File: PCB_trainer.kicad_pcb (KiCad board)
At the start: 2 copper layers, 76.7 x 55.9 mm, 6 parts, among them IC1 IS42S16800F-7BLI, U1 STM32F103C8Tx, U2 MIMXRT1062DVJ6B, U3 STM32F407VGTx, U4 MIC23158YML-T5, U5 W25Q64JVXGIQ TR

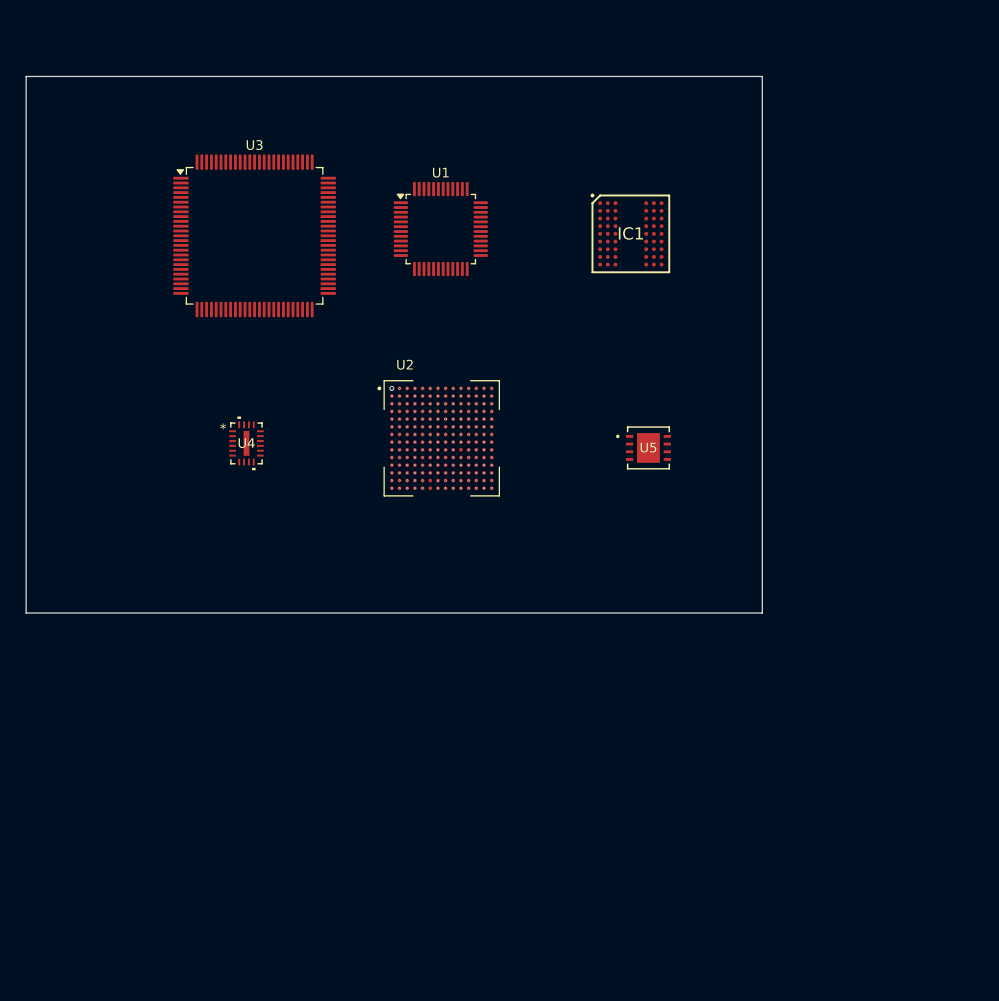
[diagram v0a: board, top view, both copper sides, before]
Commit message: finalised pcb
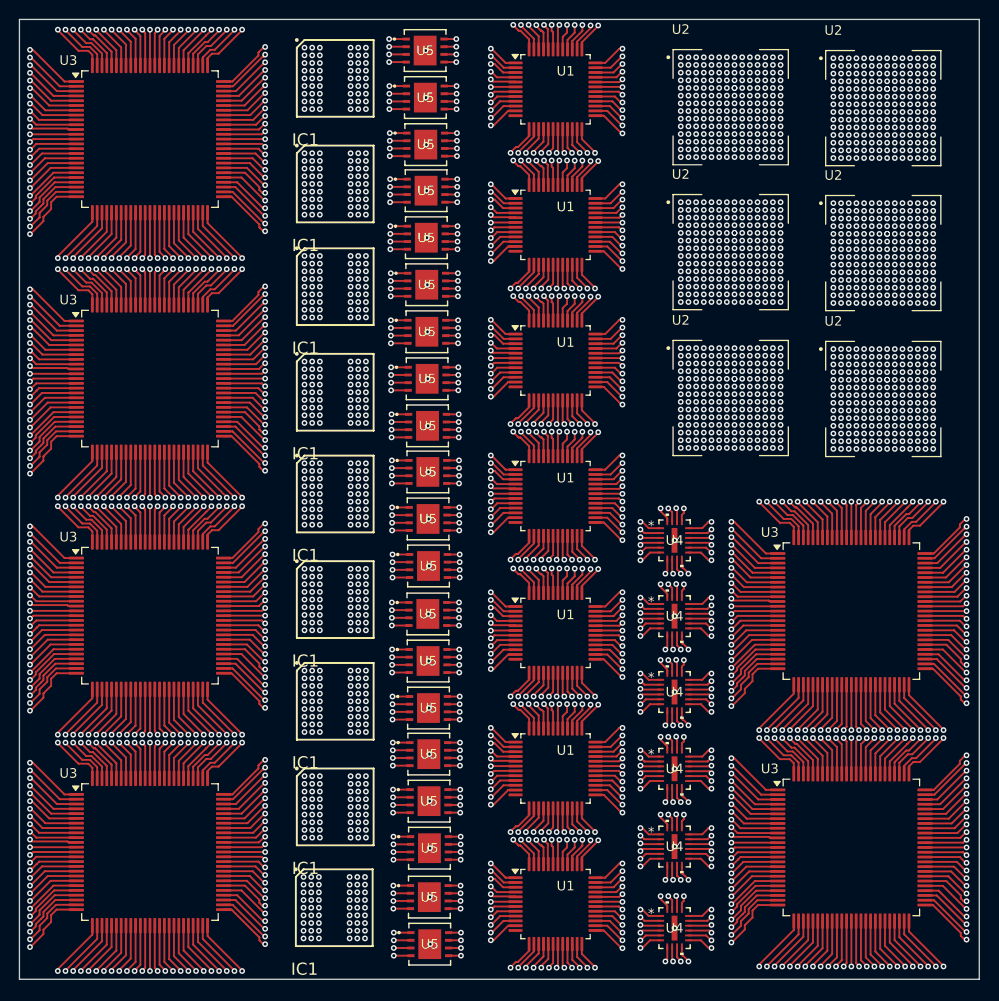
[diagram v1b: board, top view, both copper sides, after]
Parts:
- added IC1: IS42S16800F-7BLI, LIB_IS42S16800F-7BLI:BGA54C80P9X9_800X800X120, F.Cu at (132.9, 110.9)
- added IC1: IS42S16800F-7BLI, LIB_IS42S16800F-7BLI:BGA54C80P9X9_800X800X120, F.Cu at (132.9, 100.3)
- added IC1: IS42S16800F-7BLI, LIB_IS42S16800F-7BLI:BGA54C80P9X9_800X800X120, F.Cu at (132.9, 121.9)
- added IC1: IS42S16800F-7BLI, LIB_IS42S16800F-7BLI:BGA54C80P9X9_800X800X120, F.Cu at (132.9, 78.7)
- added IC1: IS42S16800F-7BLI, LIB_IS42S16800F-7BLI:BGA54C80P9X9_800X800X120, F.Cu at (132.9, 57.0)
- added IC1: IS42S16800F-7BLI, LIB_IS42S16800F-7BLI:BGA54C80P9X9_800X800X120, F.Cu at (132.9, 89.3)
- added IC1: IS42S16800F-7BLI, LIB_IS42S16800F-7BLI:BGA54C80P9X9_800X800X120, F.Cu at (132.8, 132.4)
- added IC1: IS42S16800F-7BLI, LIB_IS42S16800F-7BLI:BGA54C80P9X9_800X800X120, F.Cu at (132.9, 67.7)
- added U1: STM32F103C8Tx, Package_QFP:LQFP-48_7x7mm_P0.5mm, F.Cu at (155.8, 75.4)
- added U1: STM32F103C8Tx, Package_QFP:LQFP-48_7x7mm_P0.5mm, F.Cu at (155.8, 132.0)
- added U1: STM32F103C8Tx, Package_QFP:LQFP-48_7x7mm_P0.5mm, F.Cu at (155.8, 89.5)
- added U1: STM32F103C8Tx, Package_QFP:LQFP-48_7x7mm_P0.5mm, F.Cu at (155.8, 103.8)
- added U1: STM32F103C8Tx, Package_QFP:LQFP-48_7x7mm_P0.5mm, F.Cu at (155.8, 117.9)
- added U1: STM32F103C8Tx, Package_QFP:LQFP-48_7x7mm_P0.5mm, F.Cu at (155.8, 61.3)
- added U2: MIMXRT1062DVJ6B, MIMXRT1062DVJ6B:BGA196C80P14X14_1200X1200X152N, F.Cu at (174.1, 79.3)
- added U2: MIMXRT1062DVJ6B, MIMXRT1062DVJ6B:BGA196C80P14X14_1200X1200X152N, F.Cu at (174.1, 64.1)
- added U2: MIMXRT1062DVJ6B, MIMXRT1062DVJ6B:BGA196C80P14X14_1200X1200X152N, F.Cu at (190.0, 49.1)
- added U2: MIMXRT1062DVJ6B, MIMXRT1062DVJ6B:BGA196C80P14X14_1200X1200X152N, F.Cu at (190.0, 79.4)
- added U2: MIMXRT1062DVJ6B, MIMXRT1062DVJ6B:BGA196C80P14X14_1200X1200X152N, F.Cu at (190.0, 64.2)
- added U3: STM32F407VGTx, Package_QFP:LQFP-100_14x14mm_P0.5mm, F.Cu at (186.7, 101.5)
- added U3: STM32F407VGTx, Package_QFP:LQFP-100_14x14mm_P0.5mm, F.Cu at (186.7, 126.1)
- added U3: STM32F407VGTx, Package_QFP:LQFP-100_14x14mm_P0.5mm, F.Cu at (113.6, 126.6)
- added U3: STM32F407VGTx, Package_QFP:LQFP-100_14x14mm_P0.5mm, F.Cu at (113.6, 77.3)
- added U3: STM32F407VGTx, Package_QFP:LQFP-100_14x14mm_P0.5mm, F.Cu at (113.6, 102.0)
- added U4: MIC23158YML-T5, ul_MIC23158YML-T5:QFN20_3X4_MCH, F.Cu at (168.3, 117.9)
- added U4: MIC23158YML-T5, ul_MIC23158YML-T5:QFN20_3X4_MCH, F.Cu at (168.3, 134.5)
- added U4: MIC23158YML-T5, ul_MIC23158YML-T5:QFN20_3X4_MCH, F.Cu at (168.3, 109.9)
- added U4: MIC23158YML-T5, ul_MIC23158YML-T5:QFN20_3X4_MCH, F.Cu at (168.3, 126.0)
- added U4: MIC23158YML-T5, ul_MIC23158YML-T5:QFN20_3X4_MCH, F.Cu at (168.3, 102.0)
- added U5: W25Q64JVXGIQ TR, ul_W25Q64JVXGIQ-TR:DFN_XGIQ TR_WIN, F.Cu at (142.6, 111.6)
- added U5: W25Q64JVXGIQ TR, ul_W25Q64JVXGIQ-TR:DFN_XGIQ TR_WIN, F.Cu at (142.7, 121.3)
- added U5: W25Q64JVXGIQ TR, ul_W25Q64JVXGIQ-TR:DFN_XGIQ TR_WIN, F.Cu at (142.4, 72.4)
- added U5: W25Q64JVXGIQ TR, ul_W25Q64JVXGIQ-TR:DFN_XGIQ TR_WIN, F.Cu at (142.5, 87.0)
- added U5: W25Q64JVXGIQ TR, ul_W25Q64JVXGIQ-TR:DFN_XGIQ TR_WIN, F.Cu at (142.4, 62.6)
- added U5: W25Q64JVXGIQ TR, ul_W25Q64JVXGIQ-TR:DFN_XGIQ TR_WIN, F.Cu at (142.6, 96.8)
- added U5: W25Q64JVXGIQ TR, ul_W25Q64JVXGIQ-TR:DFN_XGIQ TR_WIN, F.Cu at (142.7, 126.2)
- added U5: W25Q64JVXGIQ TR, ul_W25Q64JVXGIQ-TR:DFN_XGIQ TR_WIN, F.Cu at (142.3, 48.0)
- added U5: W25Q64JVXGIQ TR, ul_W25Q64JVXGIQ-TR:DFN_XGIQ TR_WIN, F.Cu at (142.6, 91.9)
- added U5: W25Q64JVXGIQ TR, ul_W25Q64JVXGIQ-TR:DFN_XGIQ TR_WIN, F.Cu at (142.3, 52.9)
- added U5: W25Q64JVXGIQ TR, ul_W25Q64JVXGIQ-TR:DFN_XGIQ TR_WIN, F.Cu at (142.7, 136.2)
- added U5: W25Q64JVXGIQ TR, ul_W25Q64JVXGIQ-TR:DFN_XGIQ TR_WIN, F.Cu at (142.6, 106.7)
- added U5: W25Q64JVXGIQ TR, ul_W25Q64JVXGIQ-TR:DFN_XGIQ TR_WIN, F.Cu at (142.5, 101.8)
- added U5: W25Q64JVXGIQ TR, ul_W25Q64JVXGIQ-TR:DFN_XGIQ TR_WIN, F.Cu at (142.7, 131.3)
- added U5: W25Q64JVXGIQ TR, ul_W25Q64JVXGIQ-TR:DFN_XGIQ TR_WIN, F.Cu at (142.4, 57.7)
- added U5: W25Q64JVXGIQ TR, ul_W25Q64JVXGIQ-TR:DFN_XGIQ TR_WIN, F.Cu at (142.5, 82.2)
- added U5: W25Q64JVXGIQ TR, ul_W25Q64JVXGIQ-TR:DFN_XGIQ TR_WIN, F.Cu at (142.5, 77.3)
- added U5: W25Q64JVXGIQ TR, ul_W25Q64JVXGIQ-TR:DFN_XGIQ TR_WIN, F.Cu at (142.4, 67.5)
- added U5: W25Q64JVXGIQ TR, ul_W25Q64JVXGIQ-TR:DFN_XGIQ TR_WIN, F.Cu at (142.6, 116.4)
- moved U5 47.5 mm to (142.3, 43.1)
- moved U2 45.8 mm to (174.1, 49.0)
- moved U4 45.7 mm to (168.3, 94.1)
- moved IC1 34.8 mm to (132.9, 46.0)
- moved U1 18.8 mm to (155.8, 47.1)
- moved U3 14.8 mm to (113.6, 52.3)
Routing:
- net Net-(U3-VSS-Pad10): track 0.00 -> 134.5 mm, vias 0 -> 24
- net Net-(U1-VSS-Pad23): track 0.00 -> 65.2 mm, vias 0 -> 21
- net unconnected-(U3-PA2-Pad25): track 0.00 -> 42.8 mm, vias 0 -> 6
- net unconnected-(U3-PA1-Pad24): track 0.00 -> 41.2 mm, vias 0 -> 6
- net unconnected-(U3-PA0-Pad23): track 0.00 -> 39.6 mm, vias 0 -> 6
- net unconnected-(U3-VDDA-Pad22): track 0.00 -> 38.1 mm, vias 0 -> 6
- net unconnected-(U3-VDD-Pad50): track 0.00 -> 37.3 mm, vias 0 -> 6
- net unconnected-(U3-PA3-Pad26): track 0.00 -> 37.3 mm, vias 0 -> 6
- net unconnected-(U3-PE2-Pad1): track 0.00 -> 37.2 mm, vias 0 -> 6
- net unconnected-(U3-VCAP_1-Pad49): track 0.00 -> 36.6 mm, vias 0 -> 6
- net unconnected-(U3-VREF+-Pad21): track 0.00 -> 36.5 mm, vias 0 -> 6
- net unconnected-(U3-PE3-Pad2): track 0.00 -> 36.4 mm, vias 0 -> 6
- net unconnected-(U3-VDD-Pad75): track 0.00 -> 36.0 mm, vias 0 -> 6
- net unconnected-(U3-PB12-Pad51): track 0.00 -> 36.0 mm, vias 0 -> 6
- net unconnected-(U3-VDD-Pad28): track 0.00 -> 35.8 mm, vias 0 -> 6
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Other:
- board size 76.7 x 55.9 mm -> 100 x 100 mm
